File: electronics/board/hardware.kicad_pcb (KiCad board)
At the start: 4 copper layers, 28.5 x 20.5 mm, 25 parts, among them J1 Hirose_BM24_BM24-40DP-2-0.35V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, U1 Val**, U2 Val**, U3 Val**, U4 Val**

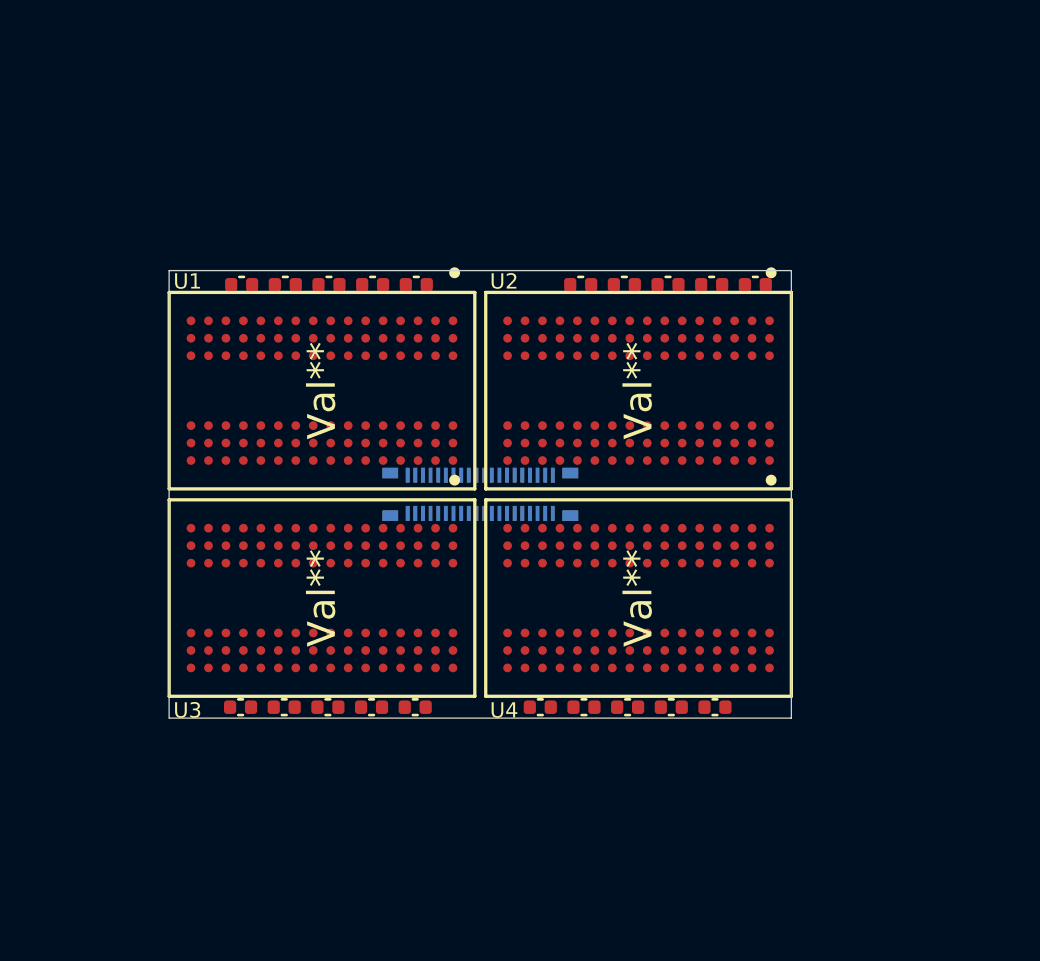
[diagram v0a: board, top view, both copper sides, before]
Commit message: Added the schematics for the rams and stuff.
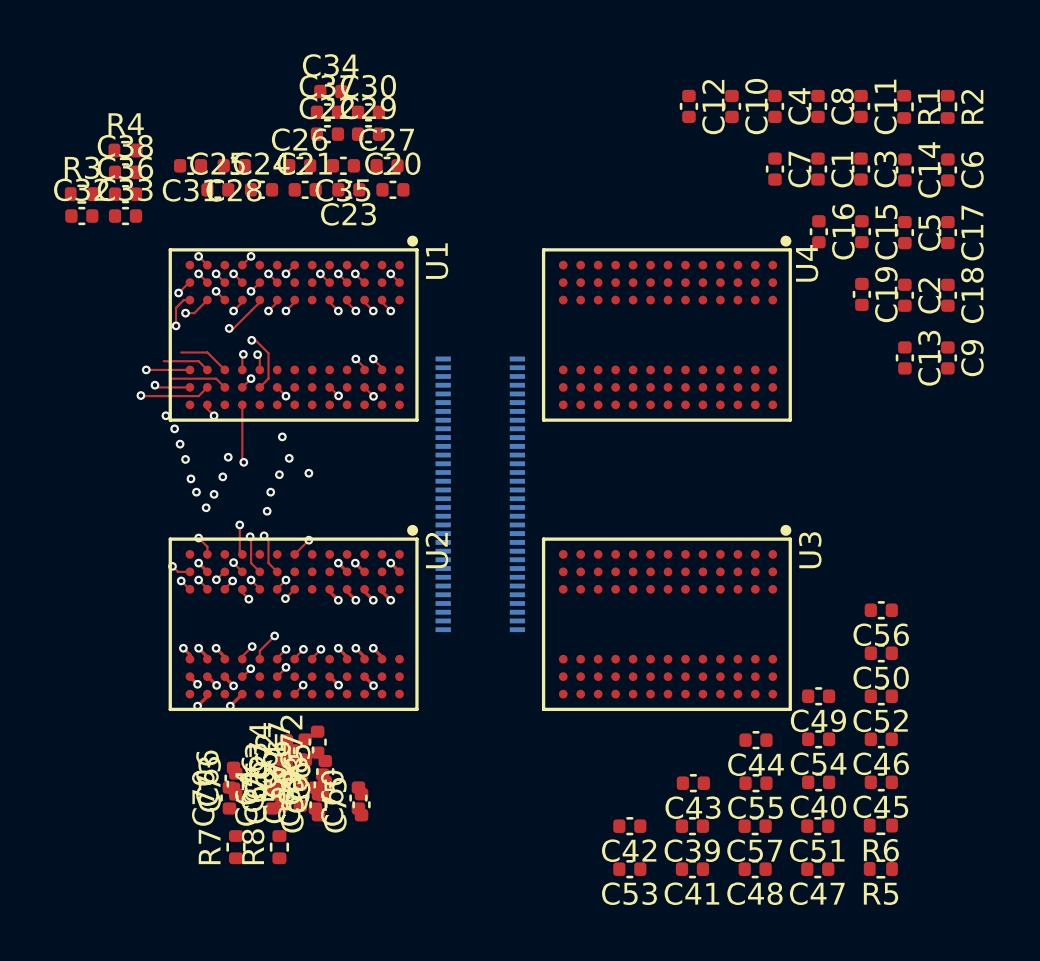
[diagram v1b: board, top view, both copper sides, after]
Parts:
- removed the C34 at (130.6, 102.9)
- removed the C34 at (115.1, 102.9)
- removed the C34 at (128.8, 122.2)
- removed the C34 at (115.0, 122.2)
- removed the C39 at (119.1, 102.9)
- removed the C39 at (119.0, 122.2)
- removed the C39 at (134.6, 102.9)
- removed the C39 at (132.8, 122.2)
- removed the C47 at (121.0, 122.2)
- removed the C47 at (134.8, 122.2)
- removed the C47 at (121.1, 102.9)
- removed the C47 at (136.6, 102.9)
- removed the C51 at (113.0, 122.2)
- removed the C51 at (128.6, 102.9)
- removed the C51 at (126.8, 122.2)
- removed the C51 at (113.1, 102.9)
- removed the C52 at (117.0, 122.2)
- removed the C52 at (130.8, 122.2)
- removed the C52 at (117.1, 102.9)
- removed the C52 at (132.6, 102.9)
- added C1: 100nF, Capacitor_SMD:C_0402_1005Metric, F.Cu at (139.5, 97.6)
- added C10: 100nF, Capacitor_SMD:C_0402_1005Metric, F.Cu at (135.5, 94.7)
- added C11: 100nF, Capacitor_SMD:C_0402_1005Metric, F.Cu at (141.4, 94.7)
- added C12: 100nF, Capacitor_SMD:C_0402_1005Metric, F.Cu at (133.6, 94.7)
- added C13: 100nF, Capacitor_SMD:C_0402_1005Metric, F.Cu at (143.4, 106.2)
- added C14: 100nF, Capacitor_SMD:C_0402_1005Metric, F.Cu at (143.4, 97.6)
- added C15: 100nF, Capacitor_SMD:C_0402_1005Metric, F.Cu at (141.5, 100.5)
- added C16: 100nF, Capacitor_SMD:C_0402_1005Metric, F.Cu at (139.5, 100.5)
- added C17: 100nF, Capacitor_SMD:C_0402_1005Metric, F.Cu at (145.4, 100.5)
- added C18: 100nF, Capacitor_SMD:C_0402_1005Metric, F.Cu at (145.4, 103.4)
- added C19: 100nF, Capacitor_SMD:C_0402_1005Metric, F.Cu at (141.5, 103.3)
- added C2: 100nF, Capacitor_SMD:C_0402_1005Metric, F.Cu at (143.4, 103.4)
- added C20: 100nF, Capacitor_SMD:C_0402_1005Metric, F.Cu at (120.0, 98.5)
- added C21: 100nF, Capacitor_SMD:C_0402_1005Metric, F.Cu at (116.0, 98.5)
- added C22: 100nF, Capacitor_SMD:C_0402_1005Metric, F.Cu at (117.0, 96.0)
- added C23: 100nF, Capacitor_SMD:C_0402_1005Metric, F.Cu at (118.0, 98.5)
- added C24: 100nF, Capacitor_SMD:C_0402_1005Metric, F.Cu at (114.0, 98.5)
- added C25: 100nF, Capacitor_SMD:C_0402_1005Metric, F.Cu at (112.0, 98.5)
- added C26: 100nF, Capacitor_SMD:C_0402_1005Metric, F.Cu at (115.7, 97.5)
- added C27: 100nF, Capacitor_SMD:C_0402_1005Metric, F.Cu at (119.7, 97.5)
- added C28: 100nF, Capacitor_SMD:C_0402_1005Metric, F.Cu at (112.7, 97.5)
- added C29: 100nF, Capacitor_SMD:C_0402_1005Metric, F.Cu at (118.9, 96.0)
- added C3: 100nF, Capacitor_SMD:C_0402_1005Metric, F.Cu at (141.4, 97.6)
- added C30: 100nF, Capacitor_SMD:C_0402_1005Metric, F.Cu at (118.9, 95.0)
- added C31: 100nF, Capacitor_SMD:C_0402_1005Metric, F.Cu at (110.7, 97.5)
- added C32: 100nF, Capacitor_SMD:C_0402_1005Metric, F.Cu at (105.8, 99.8)
- added C33: 100nF, Capacitor_SMD:C_0402_1005Metric, F.Cu at (107.8, 99.8)
- added C34: 100nF, Capacitor_SMD:C_0402_1005Metric, F.Cu at (117.2, 94.0)
- added C35: 100nF, Capacitor_SMD:C_0402_1005Metric, F.Cu at (117.7, 97.5)
- added C36: 100nF, Capacitor_SMD:C_0402_1005Metric, F.Cu at (107.8, 98.8)
- added C37: 100nF, Capacitor_SMD:C_0402_1005Metric, F.Cu at (117.0, 95.0)
- added C38: 100nF, Capacitor_SMD:C_0402_1005Metric, F.Cu at (107.8, 97.8)
- added C39: 100nF, Capacitor_SMD:C_0402_1005Metric, F.Cu at (133.7, 127.7)
- added C4: 100nF, Capacitor_SMD:C_0402_1005Metric, F.Cu at (137.5, 94.7)
- added C40: 100nF, Capacitor_SMD:C_0402_1005Metric, F.Cu at (139.5, 125.7)
- added C41: 100nF, Capacitor_SMD:C_0402_1005Metric, F.Cu at (133.7, 129.7)
- added C42: 100nF, Capacitor_SMD:C_0402_1005Metric, F.Cu at (130.8, 127.7)
- added C43: 100nF, Capacitor_SMD:C_0402_1005Metric, F.Cu at (133.8, 125.7)
- added C44: 100nF, Capacitor_SMD:C_0402_1005Metric, F.Cu at (136.6, 123.8)
- added C45: 100nF, Capacitor_SMD:C_0402_1005Metric, F.Cu at (142.4, 125.7)
- added C46: 100nF, Capacitor_SMD:C_0402_1005Metric, F.Cu at (142.4, 123.7)
- added C47: 100nF, Capacitor_SMD:C_0402_1005Metric, F.Cu at (139.5, 129.7)
- added C48: 100nF, Capacitor_SMD:C_0402_1005Metric, F.Cu at (136.6, 129.7)
- added C49: 100nF, Capacitor_SMD:C_0402_1005Metric, F.Cu at (139.5, 121.8)
- added C5: 100nF, Capacitor_SMD:C_0402_1005Metric, F.Cu at (143.4, 100.5)
- added C50: 100nF, Capacitor_SMD:C_0402_1005Metric, F.Cu at (142.4, 119.8)
- added C51: 100nF, Capacitor_SMD:C_0402_1005Metric, F.Cu at (139.5, 127.7)
- added C52: 100nF, Capacitor_SMD:C_0402_1005Metric, F.Cu at (142.4, 121.8)
- added C53: 100nF, Capacitor_SMD:C_0402_1005Metric, F.Cu at (130.8, 129.7)
- added C54: 100nF, Capacitor_SMD:C_0402_1005Metric, F.Cu at (139.5, 123.7)
- added C55: 100nF, Capacitor_SMD:C_0402_1005Metric, F.Cu at (136.6, 125.7)
- added C56: 100nF, Capacitor_SMD:C_0402_1005Metric, F.Cu at (142.4, 117.8)
- added C57: 100nF, Capacitor_SMD:C_0402_1005Metric, F.Cu at (136.6, 127.7)
- added C58: 100nF, Capacitor_SMD:C_0402_1005Metric, F.Cu at (115.8, 126.3)
- added C59: 100nF, Capacitor_SMD:C_0402_1005Metric, F.Cu at (116.6, 126.7)
- added C6: 100nF, Capacitor_SMD:C_0402_1005Metric, F.Cu at (145.4, 97.6)
- added C60: 100nF, Capacitor_SMD:C_0402_1005Metric, F.Cu at (118.4, 126.4)
- added C61: 100nF, Capacitor_SMD:C_0402_1005Metric, F.Cu at (114.9, 126.3)
- added C62: 100nF, Capacitor_SMD:C_0402_1005Metric, F.Cu at (115.4, 124.7)
- added C63: 100nF, Capacitor_SMD:C_0402_1005Metric, F.Cu at (114.9, 125.2)
- added C64: 100nF, Capacitor_SMD:C_0402_1005Metric, F.Cu at (114.5, 126.4)
- added C65: 100nF, Capacitor_SMD:C_0402_1005Metric, F.Cu at (116.9, 125.2)
- added C66: 100nF, Capacitor_SMD:C_0402_1005Metric, F.Cu at (112.7, 125.5)
- added C67: 100nF, Capacitor_SMD:C_0402_1005Metric, F.Cu at (116.0, 124.2)
- added C68: 100nF, Capacitor_SMD:C_0402_1005Metric, F.Cu at (116.8, 125.8)
- added C69: 100nF, Capacitor_SMD:C_0402_1005Metric, F.Cu at (116.5, 126.4)
- added C7: 100nF, Capacitor_SMD:C_0402_1005Metric, F.Cu at (137.5, 97.6)
- added C70: 100nF, Capacitor_SMD:C_0402_1005Metric, F.Cu at (112.5, 126.4)
- added C71: 100nF, Capacitor_SMD:C_0402_1005Metric, F.Cu at (115.8, 125.1)
- added C72: 100nF, Capacitor_SMD:C_0402_1005Metric, F.Cu at (116.5, 123.8)
- added C73: 100nF, Capacitor_SMD:C_0402_1005Metric, F.Cu at (112.8, 125.8)
- added C74: 100nF, Capacitor_SMD:C_0402_1005Metric, F.Cu at (115.1, 124.2)
- added C75: 100nF, Capacitor_SMD:C_0402_1005Metric, F.Cu at (118.6, 126.7)
- added C76: 100nF, Capacitor_SMD:C_0402_1005Metric, F.Cu at (114.8, 125.8)
- added C8: 100nF, Capacitor_SMD:C_0402_1005Metric, F.Cu at (139.5, 94.7)
- added C9: 100nF, Capacitor_SMD:C_0402_1005Metric, F.Cu at (145.4, 106.2)
- added R1: 1k, Resistor_SMD:R_0402_1005Metric, F.Cu at (143.4, 94.8)
- added R2: 1k, Resistor_SMD:R_0402_1005Metric, F.Cu at (145.4, 94.8)
- added R3: 1k, Resistor_SMD:R_0402_1005Metric, F.Cu at (105.8, 98.8)
- added R4: 1k, Resistor_SMD:R_0402_1005Metric, F.Cu at (107.8, 96.8)
- added R5: 1k, Resistor_SMD:R_0402_1005Metric, F.Cu at (142.3, 129.7)
- added R6: 1k, Resistor_SMD:R_0402_1005Metric, F.Cu at (142.3, 127.7)
- added R7: 1k, Resistor_SMD:R_0402_1005Metric, F.Cu at (112.8, 128.7)
- added R8: 1k, Resistor_SMD:R_0402_1005Metric, F.Cu at (114.8, 128.7)
- J1: value Hirose_BM24_BM24-40DP-2-0.35V_2x20_P0.35mm_PowerPin2_Vertical -> 0513386473; footprint Connector_Hirose:Hirose_BM24_BM24-40DP-2-0.35V_2x20_P0.35mm_PowerPin2_Vertical -> Molex:0513386473
- U1, U2, U3, U4: value Val** -> DDR3-78; footprint DDR3:DDR3-BGA-96-Loose -> ddr3:DDR3-BGA-78-Tightest
- moved U2 20.0 mm to (114.3, 118.5)
- moved U3 14.7 mm to (131.4, 118.5)
- moved U4 12.1 mm to (131.4, 105.2)
- moved U1 3.54 mm to (114.3, 105.2)
- turned J1 to -90 degrees
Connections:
- J1 pad 1: (no net) -> /ADR0
- J1 pad 10: (no net) -> unconnected-(J1-Pad10)
- J1 pad 11: (no net) -> unconnected-(J1-Pad11)
- J1 pad 12: (no net) -> unconnected-(J1-Pad12)
- J1 pad 13: (no net) -> unconnected-(J1-Pad13)
- J1 pad 14: (no net) -> unconnected-(J1-Pad14)
- J1 pad 15: (no net) -> unconnected-(J1-Pad15)
- J1 pad 16: (no net) -> unconnected-(J1-Pad16)
- J1 pad 17: (no net) -> unconnected-(J1-Pad17)
- J1 pad 18: (no net) -> unconnected-(J1-Pad18)
- J1 pad 19: (no net) -> unconnected-(J1-Pad19)
- J1 pad 2: (no net) -> unconnected-(J1-Pad2)
- J1 pad 20: (no net) -> unconnected-(J1-Pad20)
- J1 pad 21: (no net) -> unconnected-(J1-Pad21)
- J1 pad 22: (no net) -> unconnected-(J1-Pad22)
- J1 pad 23: (no net) -> unconnected-(J1-Pad23)
- J1 pad 24: (no net) -> unconnected-(J1-Pad24)
- J1 pad 25: (no net) -> unconnected-(J1-Pad25)
- J1 pad 26: (no net) -> unconnected-(J1-Pad26)
- J1 pad 27: (no net) -> unconnected-(J1-Pad27)
- J1 pad 28: (no net) -> unconnected-(J1-Pad28)
- J1 pad 29: (no net) -> unconnected-(J1-Pad29)
- J1 pad 3: (no net) -> unconnected-(J1-Pad3)
- J1 pad 30: (no net) -> unconnected-(J1-Pad30)
- J1 pad 31: (no net) -> unconnected-(J1-Pad31)
- J1 pad 32: (no net) -> unconnected-(J1-Pad32)
- J1 pad 33: (no net) -> unconnected-(J1-Pad33)
- J1 pad 34: (no net) -> unconnected-(J1-Pad34)
- J1 pad 35: (no net) -> unconnected-(J1-Pad35)
- J1 pad 36: (no net) -> unconnected-(J1-Pad36)
- J1 pad 37: (no net) -> unconnected-(J1-Pad37)
- J1 pad 38: (no net) -> unconnected-(J1-Pad38)
- J1 pad 39: (no net) -> unconnected-(J1-Pad39)
- J1 pad 4: (no net) -> unconnected-(J1-Pad4)
- J1 pad 40: (no net) -> unconnected-(J1-Pad40)
- J1 pad 41: (no net) -> unconnected-(J1-Pad41)
- J1 pad 42: (no net) -> unconnected-(J1-Pad42)
- J1 pad 5: (no net) -> unconnected-(J1-Pad5)
- J1 pad 6: (no net) -> unconnected-(J1-Pad6)
- J1 pad 7: (no net) -> unconnected-(J1-Pad7)
- J1 pad 8: (no net) -> unconnected-(J1-Pad8)
- J1 pad 9: (no net) -> unconnected-(J1-Pad9)
- U1 pad A1: (no net) -> GND
- U1 pad A2: (no net) -> +1V35
- U1 pad A3: (no net) -> unconnected-(U1-PadA3)
- U1 pad A7: (no net) -> /~{TDQS}
- U1 pad A8: (no net) -> GND
- U1 pad A9: (no net) -> +1V35
- U1 pad B1: (no net) -> GND
- U1 pad B2: (no net) -> GND
- U1 pad B3: (no net) -> /DQ0
- U1 pad B7: (no net) -> /TDQS
- U1 pad B8: (no net) -> GND
- U1 pad B9: (no net) -> +1V35
- U1 pad C1: (no net) -> +1V35
- U1 pad C2: (no net) -> /DQ2
- U1 pad C3: (no net) -> /DQS
- U1 pad C7: (no net) -> /DQ1
- U1 pad C8: (no net) -> /DQ3
- U1 pad C9: (no net) -> +1V35
- U1 pad D1: (no net) -> GND
- U1 pad D2: (no net) -> /DQ6
- U1 pad D3: (no net) -> /~{DQS}
- U1 pad D7: (no net) -> +1V35
- U1 pad D8: (no net) -> GND
- U1 pad D9: (no net) -> GND
- U1 pad E1: (no net) -> Net-(U1-PadE1)
- U1 pad E2: (no net) -> +1V35
- U1 pad E3: (no net) -> /DQ4
- U1 pad E7: (no net) -> /DQ7
- U1 pad E8: (no net) -> /DQ5
- U1 pad E9: (no net) -> +1V35
- U1 pad F1: (no net) -> unconnected-(U1-PadF1)
- U1 pad F2: (no net) -> GND
- U1 pad F3: (no net) -> /~{RAS}
- U1 pad F7: (no net) -> /CK
- U1 pad F8: (no net) -> GND
- U1 pad F9: (no net) -> unconnected-(U1-PadF9)
- U1 pad G1: (no net) -> /ODT
- U1 pad G2: (no net) -> +1V35
- U1 pad G3: (no net) -> /~{CAS}
- U1 pad G7: (no net) -> /~{CK}
- U1 pad G8: (no net) -> +1V35
- U1 pad G9: (no net) -> /CKE
- U1 pad H1: (no net) -> unconnected-(U1-PadH1)
- U1 pad H2: (no net) -> /~{CS}
- U1 pad H3: (no net) -> /~{WE}
- U1 pad H7: (no net) -> /ADR10
- U1 pad H8: (no net) -> /ZQ
- U1 pad H9: (no net) -> unconnected-(U1-PadH9)
- U1 pad J1: (no net) -> GND
- U1 pad J2: (no net) -> /BA0
- U1 pad J3: (no net) -> /BA2
- U1 pad J7: (no net) -> /ADR15
- U1 pad J8: (no net) -> Net-(U1-PadE1)
- U1 pad J9: (no net) -> GND
- U1 pad K1: (no net) -> +1V35
- U1 pad K2: (no net) -> /ADR3
- U1 pad K3: (no net) -> /ADR0
- U1 pad K7: (no net) -> /ADR12
- U1 pad K8: (no net) -> /BA1
- U1 pad K9: (no net) -> +1V35
- U1 pad L1: (no net) -> GND
- U1 pad L2: (no net) -> /ADR5
- U1 pad L3: (no net) -> /ADR2
- U1 pad L7: (no net) -> /ADR1
- U1 pad L8: (no net) -> /ADR4
- U1 pad L9: (no net) -> GND
- U1 pad M1: (no net) -> +1V35
- U1 pad M2: (no net) -> /ADR7
- U1 pad M3: (no net) -> /ADR9
- U1 pad M7: (no net) -> /ADR11
- U1 pad M8: (no net) -> /ADR6
- U1 pad M9: (no net) -> +1V35
- U1 pad N1: (no net) -> GND
- U1 pad N2: (no net) -> /~{RESET}
- U1 pad N3: (no net) -> /ADR13
- U1 pad N7: (no net) -> /ADR14
- U1 pad N8: (no net) -> /ADR8
- U1 pad N9: (no net) -> GND
- U2 pad A1: (no net) -> GND
- U2 pad A2: (no net) -> +1V35
- U2 pad A3: (no net) -> unconnected-(U2-PadA3)
- U2 pad A7: (no net) -> /~{TDQS}
- U2 pad A8: (no net) -> GND
- U2 pad A9: (no net) -> +1V35
- U2 pad B1: (no net) -> GND
- U2 pad B2: (no net) -> GND
- U2 pad B3: (no net) -> /DQ8
- U2 pad B7: (no net) -> /TDQS
- U2 pad B8: (no net) -> GND
- U2 pad B9: (no net) -> +1V35
- U2 pad C1: (no net) -> +1V35
- U2 pad C2: (no net) -> /DQ10
- U2 pad C3: (no net) -> /DQS
- U2 pad C7: (no net) -> /DQ9
- U2 pad C8: (no net) -> /DQ11
- U2 pad C9: (no net) -> +1V35
- U2 pad D1: (no net) -> GND
- U2 pad D2: (no net) -> /DQ14
- U2 pad D3: (no net) -> /~{DQS}
- U2 pad D7: (no net) -> +1V35
- U2 pad D8: (no net) -> GND
- U2 pad D9: (no net) -> GND
- U2 pad E1: (no net) -> Net-(C32-Pad2)
- U2 pad E2: (no net) -> +1V35
- U2 pad E3: (no net) -> /DQ12
- U2 pad E7: (no net) -> /DQ15
- U2 pad E8: (no net) -> /DQ13
- U2 pad E9: (no net) -> +1V35
- U2 pad F1: (no net) -> unconnected-(U2-PadF1)
- U2 pad F2: (no net) -> GND
- U2 pad F3: (no net) -> /~{RAS}
- U2 pad F7: (no net) -> /CK
- U2 pad F8: (no net) -> GND
- U2 pad F9: (no net) -> unconnected-(U2-PadF9)
- U2 pad G1: (no net) -> /ODT
- U2 pad G2: (no net) -> +1V35
- U2 pad G3: (no net) -> /~{CAS}
- U2 pad G7: (no net) -> /~{CK}
- U2 pad G8: (no net) -> +1V35
- U2 pad G9: (no net) -> /CKE
- U2 pad H1: (no net) -> unconnected-(U2-PadH1)
- U2 pad H2: (no net) -> /~{CS}
- U2 pad H3: (no net) -> /~{WE}
- U2 pad H7: (no net) -> /ADR10
- U2 pad H8: (no net) -> /ZQ
- U2 pad H9: (no net) -> unconnected-(U2-PadH9)
- U2 pad J1: (no net) -> GND
- U2 pad J2: (no net) -> /BA0
- U2 pad J3: (no net) -> /BA2
- U2 pad J7: (no net) -> /ADR15
- U2 pad J8: (no net) -> Net-(C32-Pad2)
- U2 pad J9: (no net) -> GND
- U2 pad K1: (no net) -> +1V35
- U2 pad K2: (no net) -> /ADR3
- U2 pad K3: (no net) -> /ADR0
- U2 pad K7: (no net) -> /ADR12
- U2 pad K8: (no net) -> /BA1
- U2 pad K9: (no net) -> +1V35
- U2 pad L1: (no net) -> GND
- U2 pad L2: (no net) -> /ADR5
- U2 pad L3: (no net) -> /ADR2
- U2 pad L7: (no net) -> /ADR1
- U2 pad L8: (no net) -> /ADR4
- U2 pad L9: (no net) -> GND
- U2 pad M1: (no net) -> +1V35
- U2 pad M2: (no net) -> /ADR7
- U2 pad M3: (no net) -> /ADR9
- U2 pad M7: (no net) -> /ADR11
- U2 pad M8: (no net) -> /ADR6
- U2 pad M9: (no net) -> +1V35
- U2 pad N1: (no net) -> GND
- U2 pad N2: (no net) -> /~{RESET}
- U2 pad N3: (no net) -> /ADR13
- U2 pad N7: (no net) -> /ADR14
- U2 pad N8: (no net) -> /ADR8
- U2 pad N9: (no net) -> GND
- U3 pad A1: (no net) -> GND
- U3 pad A2: (no net) -> +1V35
- U3 pad A3: (no net) -> unconnected-(U3-PadA3)
- U3 pad A7: (no net) -> /~{TDQS}
- U3 pad A8: (no net) -> GND
- U3 pad A9: (no net) -> +1V35
- U3 pad B1: (no net) -> GND
- U3 pad B2: (no net) -> GND
- U3 pad B3: (no net) -> /ddr3_c/DQ8
- U3 pad B7: (no net) -> /TDQS
- U3 pad B8: (no net) -> GND
- U3 pad B9: (no net) -> +1V35
- U3 pad C1: (no net) -> +1V35
- U3 pad C2: (no net) -> /ddr3_c/DQ10
- U3 pad C3: (no net) -> /DQS
- U3 pad C7: (no net) -> /ddr3_c/DQ9
- U3 pad C8: (no net) -> /ddr3_c/DQ11
- U3 pad C9: (no net) -> +1V35
- U3 pad D1: (no net) -> GND
- U3 pad D2: (no net) -> /ddr3_c/DQ14
- U3 pad D3: (no net) -> /~{DQS}
- U3 pad D7: (no net) -> +1V35
- U3 pad D8: (no net) -> GND
- U3 pad D9: (no net) -> GND
- U3 pad E1: (no net) -> Net-(C51-Pad2)
- U3 pad E2: (no net) -> +1V35
- U3 pad E3: (no net) -> /ddr3_c/DQ12
- U3 pad E7: (no net) -> /ddr3_c/DQ15
- U3 pad E8: (no net) -> /ddr3_c/DQ13
- U3 pad E9: (no net) -> +1V35
- U3 pad F1: (no net) -> unconnected-(U3-PadF1)
- U3 pad F2: (no net) -> GND
- U3 pad F3: (no net) -> /~{RAS}
- U3 pad F7: (no net) -> /CK
- U3 pad F8: (no net) -> GND
- U3 pad F9: (no net) -> unconnected-(U3-PadF9)
- U3 pad G1: (no net) -> /ODT
- U3 pad G2: (no net) -> +1V35
- U3 pad G3: (no net) -> /~{CAS}
- U3 pad G7: (no net) -> /~{CK}
- U3 pad G8: (no net) -> +1V35
- U3 pad G9: (no net) -> /CKE
- U3 pad H1: (no net) -> unconnected-(U3-PadH1)
- U3 pad H2: (no net) -> /~{CS}
- U3 pad H3: (no net) -> /~{WE}
- U3 pad H7: (no net) -> /ADR10
- U3 pad H8: (no net) -> /ZQ
- U3 pad H9: (no net) -> unconnected-(U3-PadH9)
- U3 pad J1: (no net) -> GND
- U3 pad J2: (no net) -> /BA0
- U3 pad J3: (no net) -> /BA2
- U3 pad J7: (no net) -> /ADR15
- U3 pad J8: (no net) -> Net-(C51-Pad2)
- U3 pad J9: (no net) -> GND
- U3 pad K1: (no net) -> +1V35
- U3 pad K2: (no net) -> /ADR3
- U3 pad K3: (no net) -> /ADR0
- U3 pad K7: (no net) -> /ADR12
- U3 pad K8: (no net) -> /BA1
- U3 pad K9: (no net) -> +1V35
- U3 pad L1: (no net) -> GND
- U3 pad L2: (no net) -> /ADR5
- U3 pad L3: (no net) -> /ADR2
- U3 pad L7: (no net) -> /ADR1
- U3 pad L8: (no net) -> /ADR4
- U3 pad L9: (no net) -> GND
- U3 pad M1: (no net) -> +1V35
- U3 pad M2: (no net) -> /ADR7
- U3 pad M3: (no net) -> /ADR9
- U3 pad M7: (no net) -> /ADR11
- U3 pad M8: (no net) -> /ADR6
- U3 pad M9: (no net) -> +1V35
- U3 pad N1: (no net) -> GND
- U3 pad N2: (no net) -> /~{RESET}
- U3 pad N3: (no net) -> /ADR13
- U3 pad N7: (no net) -> /ADR14
- U3 pad N8: (no net) -> /ADR8
- U3 pad N9: (no net) -> GND
- U4 pad A1: (no net) -> GND
- U4 pad A2: (no net) -> +1V35
- U4 pad A3: (no net) -> unconnected-(U4-PadA3)
- U4 pad A7: (no net) -> /~{TDQS}
- U4 pad A8: (no net) -> GND
- U4 pad A9: (no net) -> +1V35
- U4 pad B1: (no net) -> GND
- U4 pad B2: (no net) -> GND
- U4 pad B3: (no net) -> /DQ8
- U4 pad B7: (no net) -> /TDQS
- U4 pad B8: (no net) -> GND
- U4 pad B9: (no net) -> +1V35
- U4 pad C1: (no net) -> +1V35
- U4 pad C2: (no net) -> /DQ10
- U4 pad C3: (no net) -> /DQS
- U4 pad C7: (no net) -> /DQ9
- U4 pad C8: (no net) -> /DQ11
- U4 pad C9: (no net) -> +1V35
- U4 pad D1: (no net) -> GND
- U4 pad D2: (no net) -> /DQ14
- U4 pad D3: (no net) -> /~{DQS}
- U4 pad D7: (no net) -> +1V35
- U4 pad D8: (no net) -> GND
- U4 pad D9: (no net) -> GND
- U4 pad E1: (no net) -> Net-(C70-Pad2)
- U4 pad E2: (no net) -> +1V35
- U4 pad E3: (no net) -> /DQ12
- U4 pad E7: (no net) -> /DQ15
- U4 pad E8: (no net) -> /DQ13
- U4 pad E9: (no net) -> +1V35
- U4 pad F1: (no net) -> unconnected-(U4-PadF1)
- U4 pad F2: (no net) -> GND
- U4 pad F3: (no net) -> /~{RAS}
- U4 pad F7: (no net) -> /CK
- U4 pad F8: (no net) -> GND
- U4 pad F9: (no net) -> unconnected-(U4-PadF9)
- U4 pad G1: (no net) -> /ODT
- U4 pad G2: (no net) -> +1V35
- U4 pad G3: (no net) -> /~{CAS}
- U4 pad G7: (no net) -> /~{CK}
- U4 pad G8: (no net) -> +1V35
- U4 pad G9: (no net) -> /CKE
- U4 pad H1: (no net) -> unconnected-(U4-PadH1)
- U4 pad H2: (no net) -> /~{CS}
- U4 pad H3: (no net) -> /~{WE}
- U4 pad H7: (no net) -> /ADR10
- U4 pad H8: (no net) -> /ZQ
- U4 pad H9: (no net) -> unconnected-(U4-PadH9)
- U4 pad J1: (no net) -> GND
- U4 pad J2: (no net) -> /BA0
- U4 pad J3: (no net) -> /BA2
- U4 pad J7: (no net) -> /ADR15
- U4 pad J8: (no net) -> Net-(C70-Pad2)
- U4 pad J9: (no net) -> GND
- U4 pad K1: (no net) -> +1V35
- U4 pad K2: (no net) -> /ADR3
- U4 pad K3: (no net) -> /ADR0
- U4 pad K7: (no net) -> /ADR12
- U4 pad K8: (no net) -> /BA1
- U4 pad K9: (no net) -> +1V35
- U4 pad L1: (no net) -> GND
- U4 pad L2: (no net) -> /ADR5
- U4 pad L3: (no net) -> /ADR2
- U4 pad L7: (no net) -> /ADR1
- U4 pad L8: (no net) -> /ADR4
- U4 pad L9: (no net) -> GND
- U4 pad M1: (no net) -> +1V35
- U4 pad M2: (no net) -> /ADR7
- U4 pad M3: (no net) -> /ADR9
- U4 pad M7: (no net) -> /ADR11
- U4 pad M8: (no net) -> /ADR6
- U4 pad M9: (no net) -> +1V35
- U4 pad N1: (no net) -> GND
- U4 pad N2: (no net) -> /~{RESET}
- U4 pad N3: (no net) -> /ADR13
- U4 pad N7: (no net) -> /ADR14
- U4 pad N8: (no net) -> /ADR8
- U4 pad N9: (no net) -> GND
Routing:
- net /ADR5: track 0.00 -> 19.3 mm, vias 0 -> 3
- net /~{RESET}: track 0.00 -> 18.8 mm, vias 0 -> 3
- net /ADR7: track 0.00 -> 18.3 mm, vias 0 -> 3
- net /ADR9: track 0.00 -> 18.2 mm, vias 0 -> 3
- net /ADR13: track 0.00 -> 17.9 mm, vias 0 -> 3
- net /ADR2: track 0.00 -> 17.6 mm, vias 0 -> 3
- net /ADR0: track 0.00 -> 16.3 mm, vias 0 -> 3
- net /BA0: track 0.00 -> 16.2 mm, vias 0 -> 3
- net /BA2: track 0.00 -> 16.0 mm, vias 0 -> 3
- net /ADR12: track 0.00 -> 15.9 mm, vias 0 -> 3
- net /~{CS}: track 0.00 -> 15.8 mm, vias 0 -> 2
- net /ADR15: track 0.00 -> 15.8 mm, vias 0 -> 3
- net /ADR3: track 0.00 -> 15.7 mm, vias 0 -> 3
- net /BA1: track 0.00 -> 15.5 mm, vias 0 -> 3
- net /~{CAS}: track 0.00 -> 15.3 mm, vias 0 -> 3
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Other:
- board outline removed
- copper layers 4 -> 6
